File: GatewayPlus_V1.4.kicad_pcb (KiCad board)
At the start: 2 copper layers, 100 x 60 mm, 276 parts, among them IC1 MP1584EN, IC2 MP1584EN, J1 SWD_LOG, J10 USB_OTG, J11 USB_WIFI, J2 LTDC_LCD_FPC_40p, J3 Micro_SD_Card, J4 ESP Anten, J5 LoRa_Anten, J6 HR911105A, J7 RS485, J8 Conn_Jack-DC, J9 AudioJack, Q1 BC847, Q2 BC847, SW1 SW_Push, SW2 ESP_RESET, SW3 ESP_BOOT, U1 STM32F429IGTx, U10 USBLC6-2SC6, U11 USBLC6-2SC6, U2 IS42S16400J - HY57V641620E, U3 ESP32-C3, U4 W25Q32JVSS, U5 SX1278, U6 MASWSS0192, U7 LAN8720A, U8 MAX485E, U9 ES8388, Y1 25MHz, Y2 40MHz, Y3 32MHz, Y4 25MHz, Y5 32.768KHz

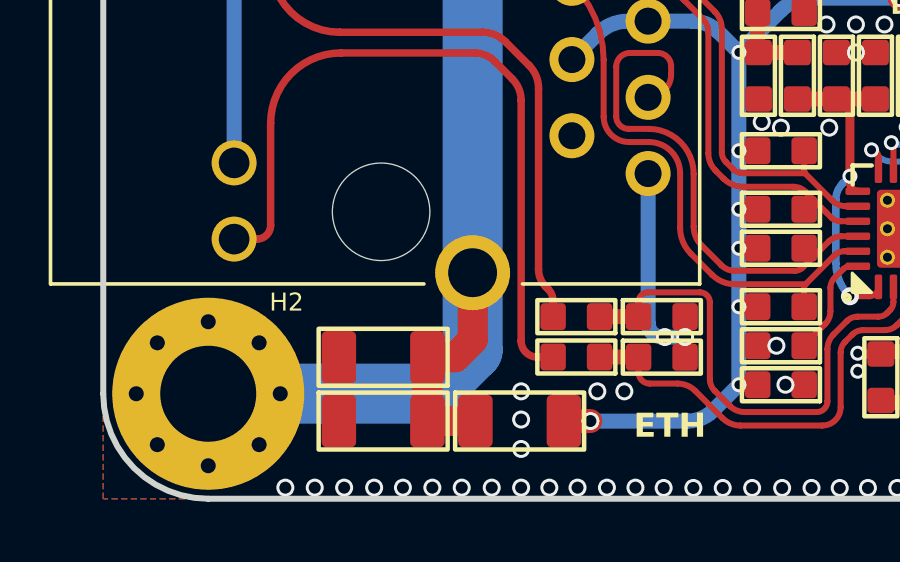
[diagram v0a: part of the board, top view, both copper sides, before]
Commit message: Finished Board.
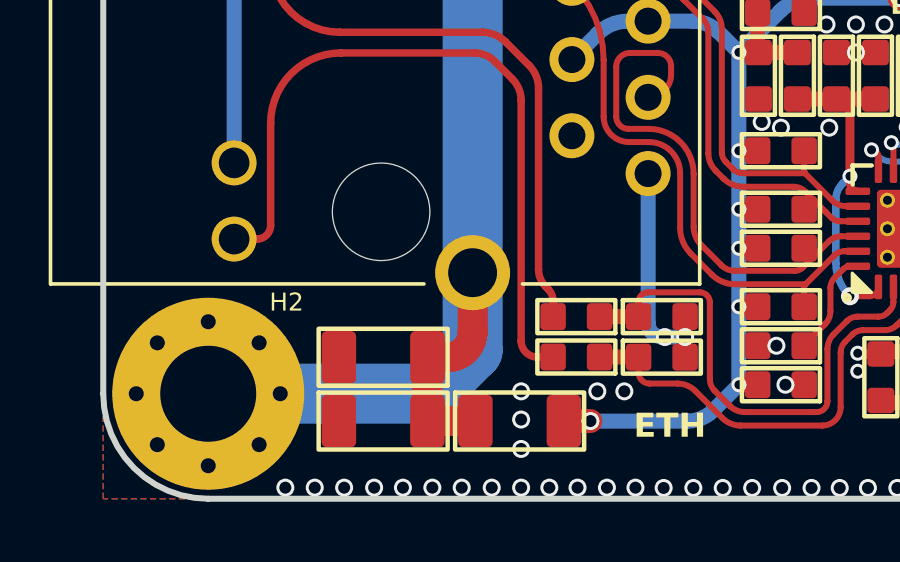
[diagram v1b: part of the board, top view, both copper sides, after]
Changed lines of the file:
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@@
   (arc (start 72.7 109) (mid 72.905061 108.915061) (end 72.99 108.71) (width 0.2) (layer "F.Cu") (net 261))
   (arc (start 71.19 109.34) (mid 71.289584 109.099584) (end 71.53 109) (width 0.2) (layer "F.Cu") (net 261))
+  (segment (start 54.155 116.685) (end 54.823219 116.685) (width 1) (layer "F.Cu") (net 263))
   (segment (start 54.155 116.685) (end 54.155 118.81) (width 1) (layer "F.Cu") (net 263))
-  (segment (start 55.6625 116.1075) (end 55.085 116.685) (width 1) (layer "F.Cu") (net 263))
-  (segment (start 55.085 116.685) (end 54.155 116.685) (width 1) (layer "F.Cu") (net 263))
   (segment (start 54.155 118.81) (end 55.755 118.81) (width 1) (layer "F.Cu") (net 263))
-  (segment (start 55.6625 113.865) (end 55.6625 116.1075) (width 1) (layer "F.Cu") (net 263))
+  (segment (start 55.6625 113.865) (end 55.6625 115.845719) (width 1) (layer "F.Cu") (net 263))
+  (arc (start 55.6625 115.845719) (mid 55.41668 116.43918) (end 54.823219 116.685) (width 1) (layer "F.Cu") (net 263))
   (segment (start 54.21 117.9) (end 46.85 117.9) (width 2) (layer "B.Cu") (net 263))
   (segment (start 55.6625 98.375) (end 55.6625 113.865) (width 2) (layer "B.Cu") (net 263))
